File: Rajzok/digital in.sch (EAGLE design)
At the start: 17 parts, among them Q1 TP0602N2, Q2 TP0602N2, Q3 SUP75N06-08, Q4 SUP75N06-08

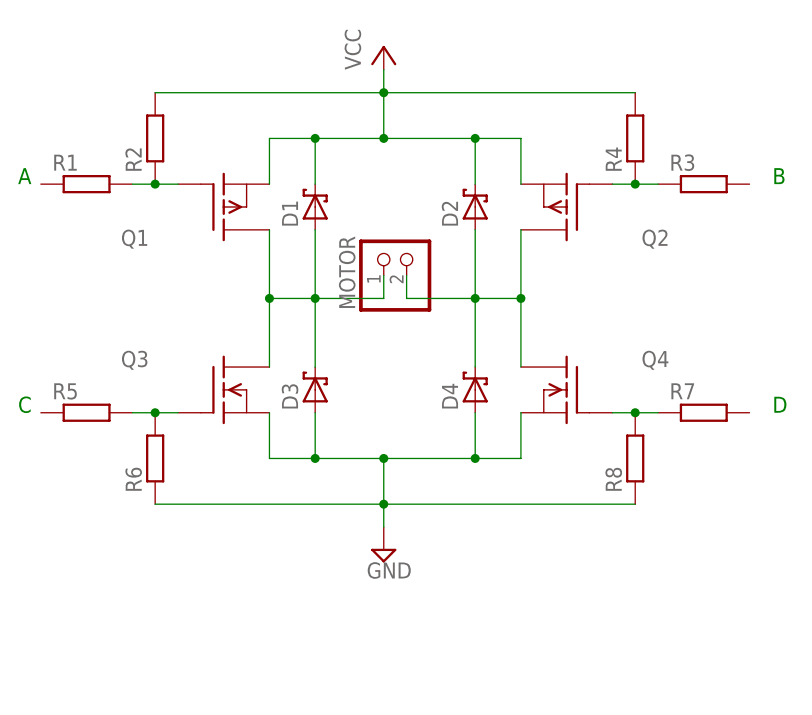
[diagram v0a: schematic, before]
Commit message: Rajzok 2017
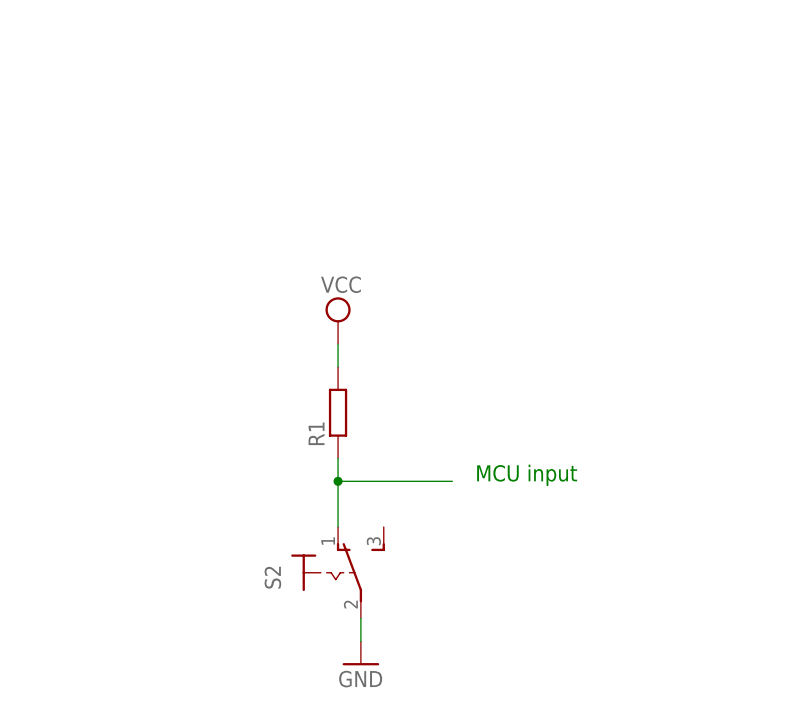
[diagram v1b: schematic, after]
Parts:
- removed D1, D2, D3, D4: 1N6267A, diode:1N6267A
- removed MOTOR: (no value), pinhead:PINHD-1X2
- removed Q1, Q2: TP0602N2, transistor-fet:TP0602N2
- removed Q3, Q4: SUP75N06-08, transistor-fet:SUP75N06-08
- removed R2, R3, R4, R5, R6, R7, R8: (no value), rcl:R-EU_0204/7
- added S2: (no value), switch:M9040P
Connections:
- removed net N$2: D2.A, D4.C, MOTOR.2, Q2.D, Q4.D
- removed net N$3: Q2.G, R3.1, R4.1
- removed net N$4: Q3.G, R5.2, R6.2
- removed net N$5: Q4.G, R7.1, R8.2
- removed net N$9: D1.A, D3.C, MOTOR.1, Q1.D, Q3.D
- net GND: now also S2.P; no longer D3.A, D4.A, Q3.S, Q4.S, R6.1, R8.1
- net N$1: now also R1.1, S2.O; no longer Q1.G, R1.2, R2.1
- net VCC: now also R1.2; no longer D1.C, D2.C, Q1.S, Q2.S, R2.2, R4.2
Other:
- note added: "MCU input"
- note removed: "A"
- note removed: "B"
- note removed: "C"
- note removed: "D"
- moved on the sheet: R1
